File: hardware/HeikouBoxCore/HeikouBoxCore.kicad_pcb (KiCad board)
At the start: 2 copper layers, 40 x 40 mm, 35 parts, among them J1 L, J2 B, J3 R, J4 T, U1 EP3C25E144

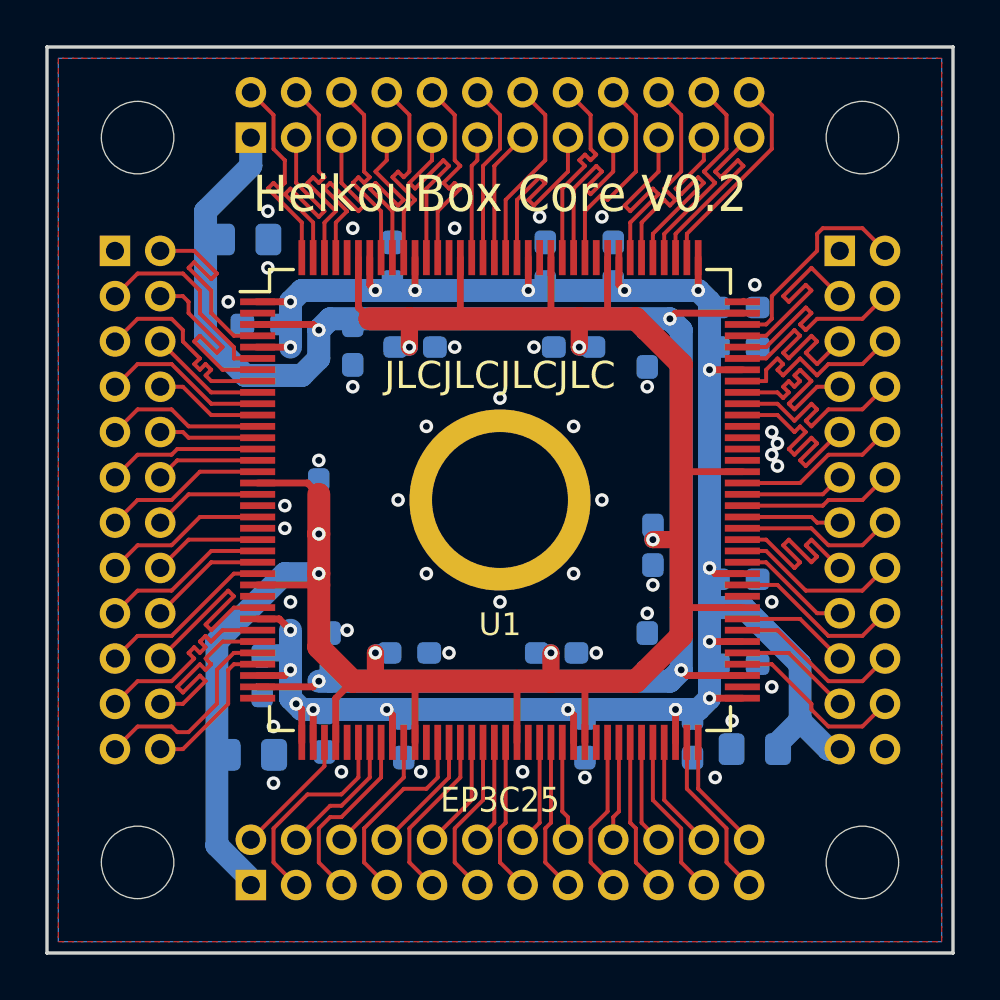
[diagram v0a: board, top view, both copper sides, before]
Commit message: Update 3D packages
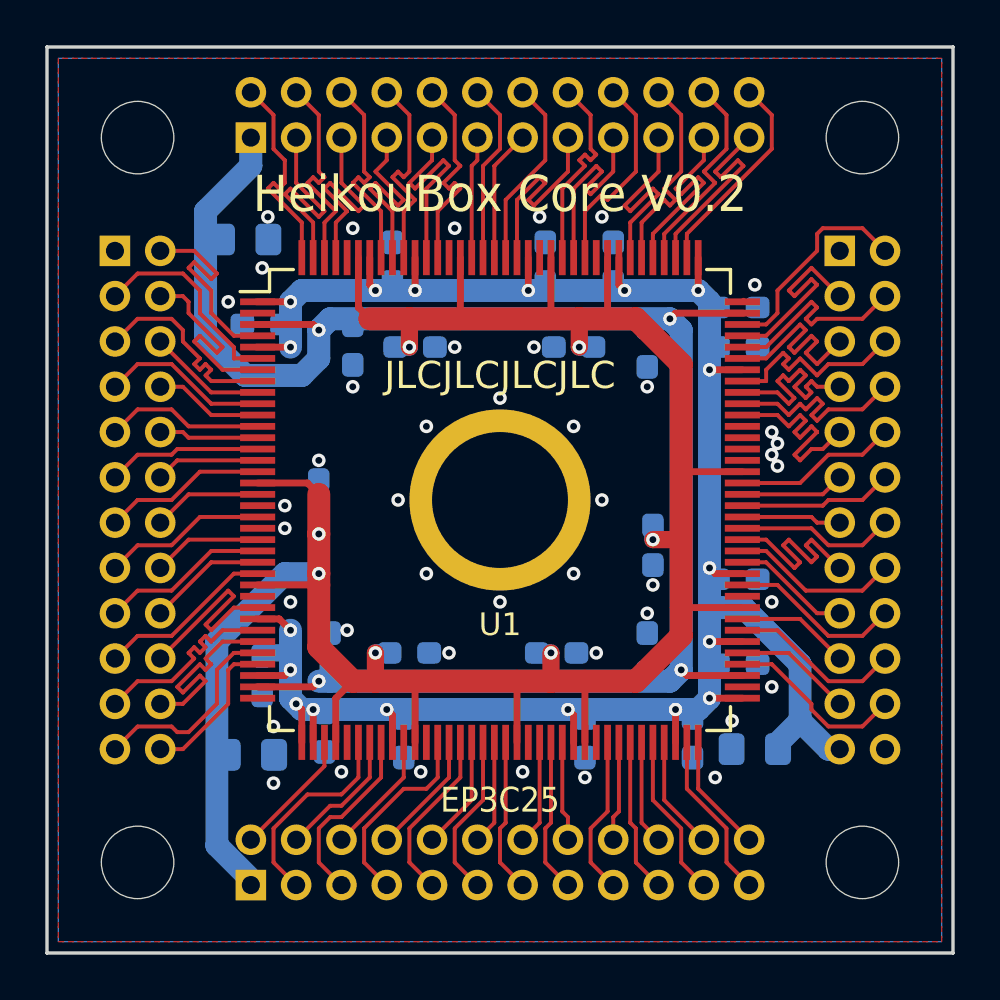
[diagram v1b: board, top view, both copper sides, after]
